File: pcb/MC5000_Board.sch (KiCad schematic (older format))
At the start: 0 parts

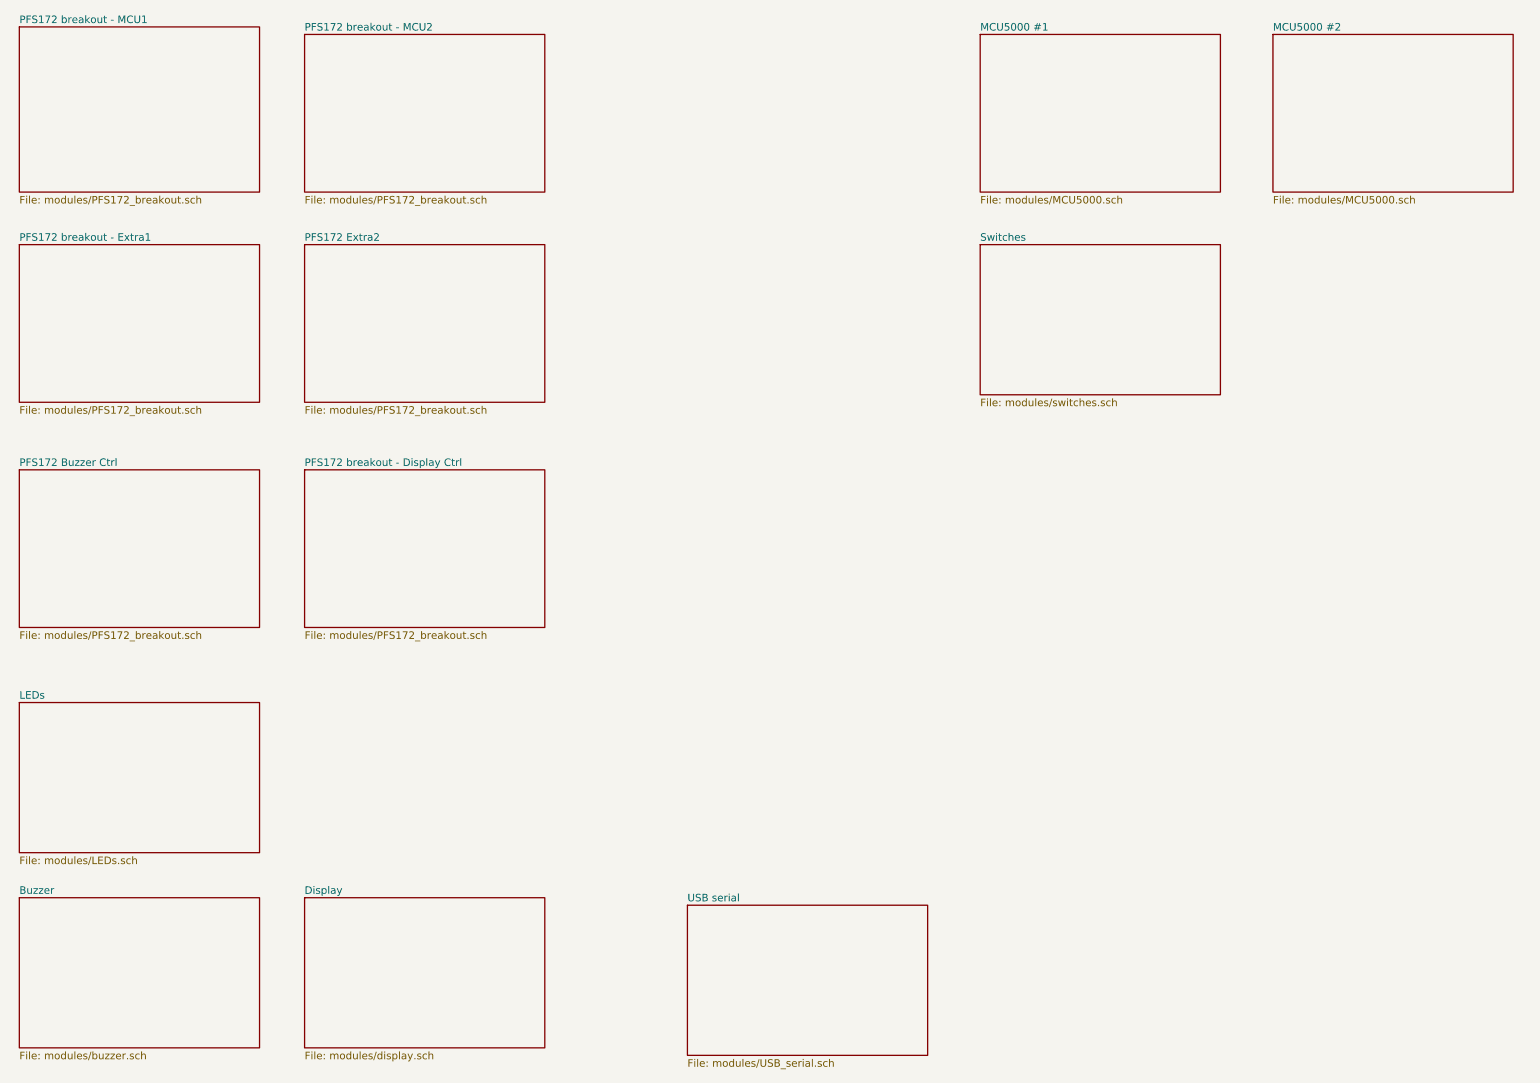
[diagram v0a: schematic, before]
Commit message: finished pcb
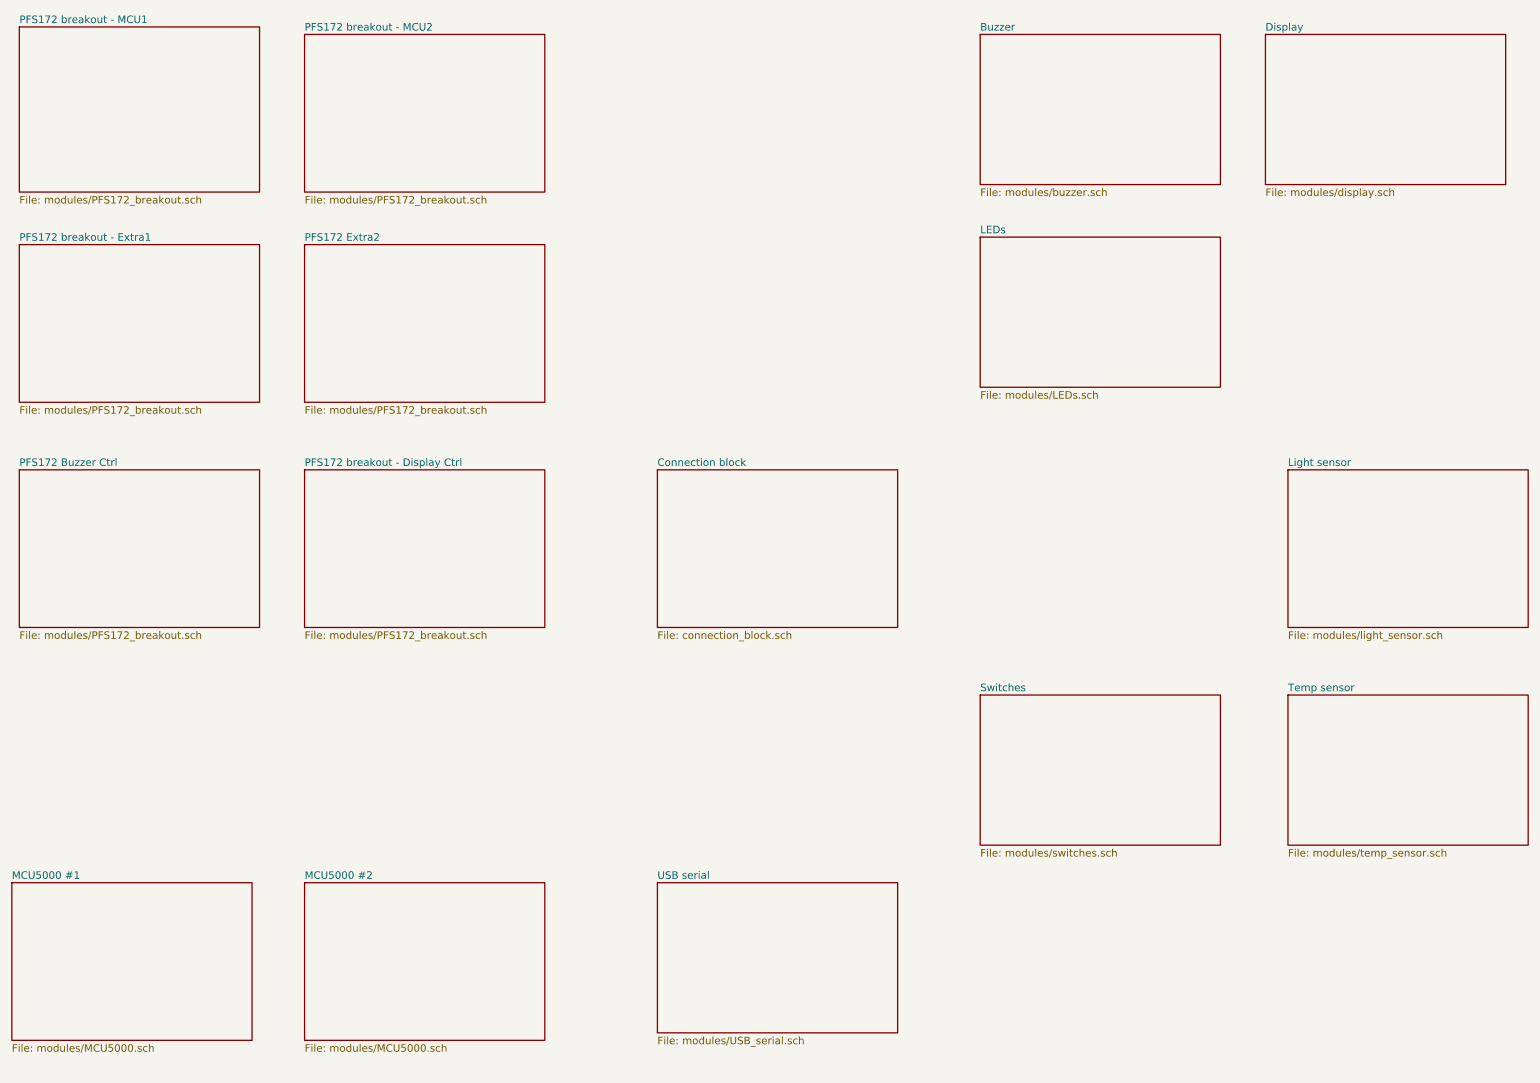
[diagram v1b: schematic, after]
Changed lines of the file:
@@
 $Descr A4 11693 8268
 encoding utf-8
-Sheet 1 14
+Sheet 1 17
 Title ""
 Date ""
@@
 $EndDescr
 $Sheet
-S 5200 6600 1600 1000
+S 5000 6450 1600 1000
 U 602FF29A
 F0 "USB serial" 50
@@
 $EndSheet
 $Sheet
-S 2650 6550 1600 1000
+S 9050 800  1600 1000
 U 60308700
 F0 "Display" 50
@@
 $EndSheet
 $Sheet
-S 7150 800  1600 1050
+S 700  6450 1600 1050
 U 6034DF24
 F0 "MCU5000 #1" 50
@@
 $EndSheet
 $Sheet
-S 9100 800  1600 1050
+S 2650 6450 1600 1050
 U 603599D1
 F0 "MCU5000 #2" 50
@@
 $EndSheet
 $Sheet
-S 750  6550 1600 1000
+S 7150 800  1600 1000
 U 603632C9
 F0 "Buzzer" 50
@@
 $EndSheet
 $Sheet
-S 750  5250 1600 1000
+S 7150 2150 1600 1000
 U 6036720E
 F0 "LEDs" 50
@@
 $EndSheet
 $Sheet
-S 7150 2200 1600 1000
+S 7150 5200 1600 1000
 U 6037B4F8
 F0 "Switches" 50
 F1 "modules/switches.sch" 50
 $EndSheet
+$Sheet
+S 9200 5200 1600 1000
+U 6038A837
+F0 "Temp sensor" 50
+F1 "modules/temp_sensor.sch" 50
+$EndSheet
+$Sheet
+S 9200 3700 1600 1050
+U 6038ECB3
+F0 "Light sensor" 50
+F1 "modules/light_sensor.sch" 50
+$EndSheet
+$Sheet
+S 5000 3700 1600 1050
+U 603839E8
+F0 "Connection block" 50
+F1 "connection_block.sch" 50
+$EndSheet
 $EndSCHEMATC
